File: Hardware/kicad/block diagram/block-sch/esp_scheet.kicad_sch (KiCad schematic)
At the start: 1 part, among them U7 ESP8266-12E_ESP-12E

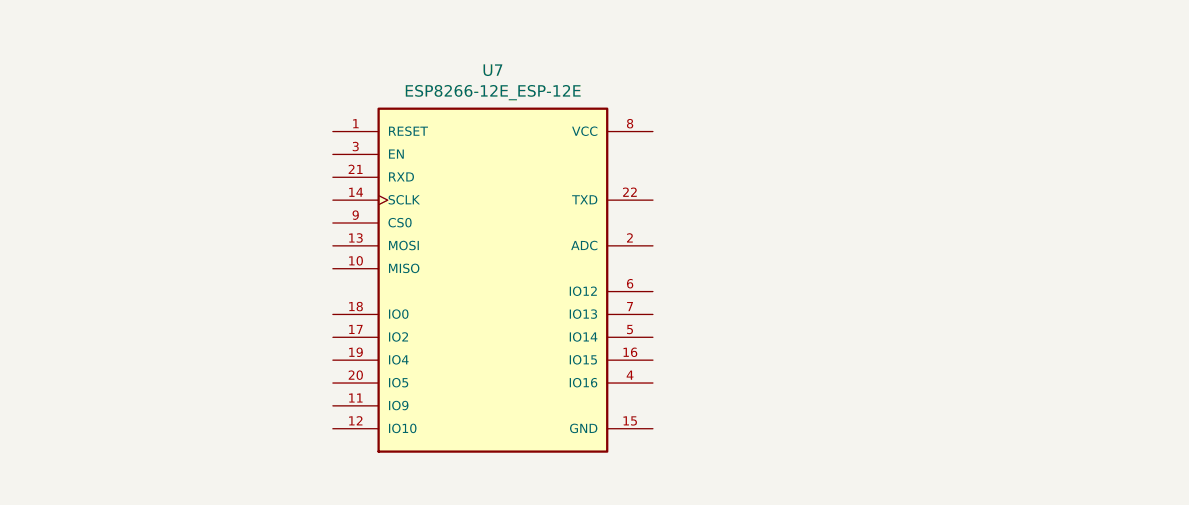
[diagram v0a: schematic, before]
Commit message: new
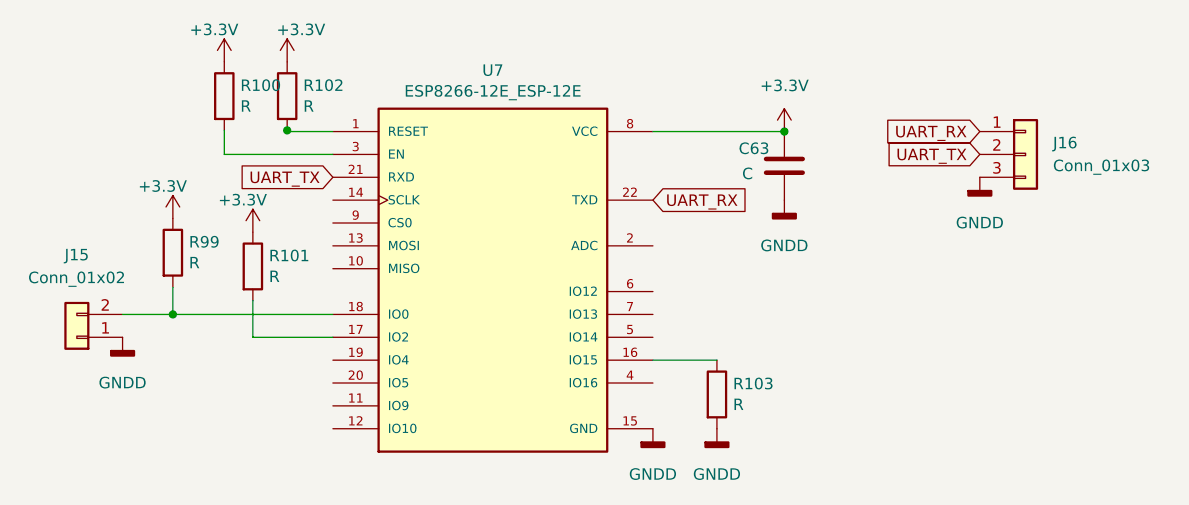
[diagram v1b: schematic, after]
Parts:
- added C63: C, Capacitor_SMD:C_0805_2012Metric, symbol Device:C
- added J15: Conn_01x02, Connector_PinHeader_1.27mm:PinHeader_1x02_P1.27mm_Vertical, symbol Connector_Generic:Conn_01x02
- added J16: Conn_01x03, Connector_PinHeader_1.27mm:PinHeader_1x03_P1.27mm_Vertical, symbol Connector_Generic:Conn_01x03
- added R100, R101, R102, R103, R99: R, Resistor_SMD:R_0805_2012Metric, symbol Device:R
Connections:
- net at U7.1 (RESET): now also R102.2
- net GNDD: now reaches U7.15 (GND)
- net GNDD: now also C63.2, J15.1 (Pin_1), J16.3 (Pin_3), R103.2
- net at U7.16 (IO15): now also R103.1
- net at U7.17 (IO2): now also R101.2
- net at U7.18 (IO0): now also J15.2 (Pin_2), R99.2
- net UART_TX: now reaches U7.21 (RXD)
- net UART_TX: now also J16.2 (Pin_2)
- net UART_RX: now reaches U7.22 (TXD)
- net UART_RX: now also J16.1 (Pin_1)
- net at U7.3 (EN): now also R100.2
- net +3V3: now reaches U7.8 (VCC)
- net +3V3: now also C63.1, R100.1, R101.1, R102.1, R99.1
